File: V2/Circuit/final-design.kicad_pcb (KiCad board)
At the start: 2 copper layers, 62.8 x 62.2 mm, 27 parts, among them J1 Conn_02x05_Odd_Even, U1 LM338T, U2 TMC2209_SILENTSTEPSTICK

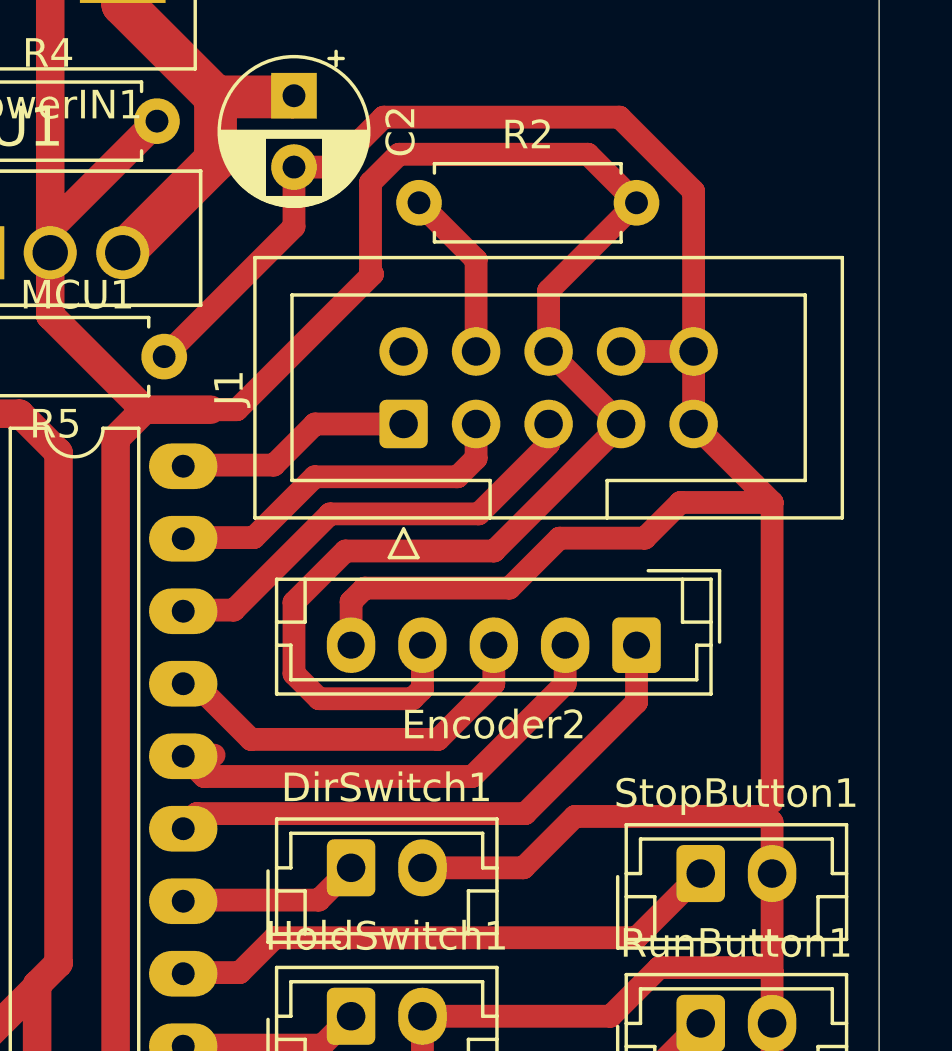
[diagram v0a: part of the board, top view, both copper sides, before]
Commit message: minor circuit changes
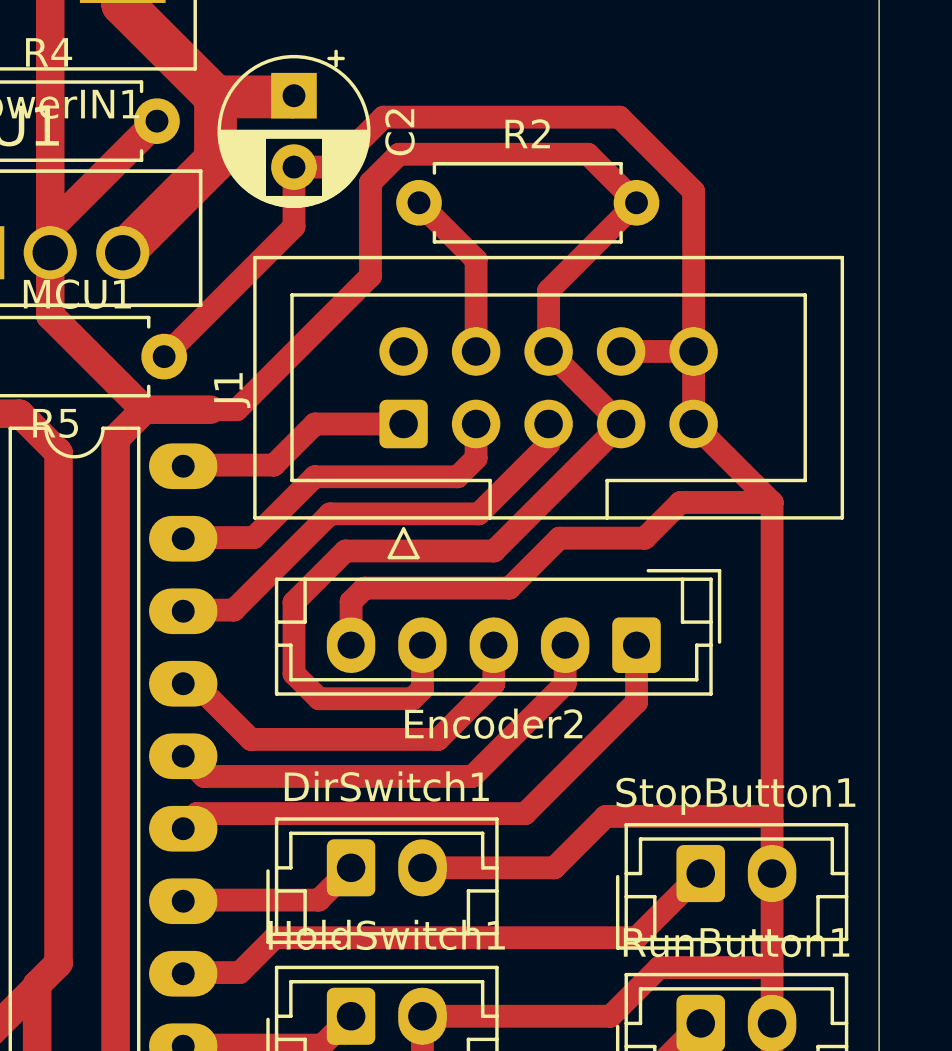
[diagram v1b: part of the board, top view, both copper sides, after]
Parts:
- R4: value 200 -> 150
- R5: value 330 -> 470
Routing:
- net Encoder_DT2: track 17.3 -> 16.2 mm
- net GND: track 356.7 -> 357.4 mm
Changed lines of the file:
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@@
 			)
 		)
-		(property "Value" "200"
+		(property "Value" "150"
 			(at 5.31 0 0)
 			(layer "F.Fab")
@@
 		)
 		(property "Value" "STC8H8K64U_SKDIP28"
-			(at 0.1 -21 0)
+			(at 0 0 90)
 			(unlocked yes)
 			(layer "F.Fab")
@@
 		)
 		(fp_text user "${REFERENCE}"
-			(at -0.2 -19.5 0)
+			(at 0.19 -15.99 0)
 			(unlocked yes)
 			(layer "F.Fab")
@@
 		)
 		(property "Value" "TMC2209_SILENTSTEPSTICK"
-			(at 11.05 11.115 0)
+			(at -1.15 -0.81 90)
 			(layer "F.Fab")
 			(effects
@@
 			)
 		)
-		(property "Value" "330"
+		(property "Value" "470"
 			(at 2.31 0 0)
 			(layer "F.Fab")
@@
 	)
 	(segment
-		(start 151.5 91.25)
-		(end 151.5 80.75)
-		(width 0.8)
-		(layer "F.Cu")
-		(net 1)
-	)
-	(segment
 		(start 121.529899 100.5)
 		(end 121.529899 100.499999)
@@
 	)
 	(segment
+		(start 151.3 91.75)
+		(end 145.669239 91.75)
+		(width 0.8)
+		(layer "F.Cu")
+		(net 1)
+	)
+	(segment
 		(start 146.75 114.25)
 		(end 146.25 114.75)
@@
 	)
 	(segment
-		(start 151.5 93.75)
-		(end 151.5 91.95)
+		(start 145.669239 91.75)
+		(end 143.869239 93.55)
 		(width 0.8)
 		(layer "F.Cu")
@@
 	)
 	(segment
-		(start 144.588478 91.75)
-		(end 142.788478 93.55)
-		(width 0.8)
-		(layer "F.Cu")
-		(net 1)
-	)
-	(segment
 		(start 105.916 95.166)
 		(end 104.95 94.2)
@@
 	)
 	(segment
+		(start 151.5 91.95)
+		(end 151.3 91.75)
+		(width 0.8)
+		(layer "F.Cu")
+		(net 1)
+	)
+	(segment
 		(start 119.75 113)
 		(end 122.69 113)
@@
 	)
 	(segment
+		(start 151.5 91.95)
+		(end 151.5 80.75)
+		(width 0.8)
+		(layer "F.Cu")
+		(net 1)
+	)
+	(segment
 		(start 104.05 76.34)
 		(end 105.65 74.74)
@@
 	)
 	(segment
-		(start 151.3 91.75)
-		(end 144.588478 91.75)
+		(start 134.75 69)
+		(end 136.137358 69)
 		(width 0.8)
 		(layer "F.Cu")
@@
 	)
 	(segment
-		(start 151.5 91.95)
-		(end 151.3 91.75)
+		(start 136.75 84.225)
+		(end 137.225 83.75)
 		(width 0.8)
 		(layer "F.Cu")
@@
 	)
 	(segment
-		(start 142.788478 93.55)
+		(start 143.869239 93.55)
 		(end 139.25 93.55)
 		(width 0.8)
@@
 	)
 	(segment
-		(start 134.75 69)
-		(end 136.137358 69)
-		(width 0.8)
-		(layer "F.Cu")
-		(net 1)
-	)
-	(segment
-		(start 136.75 84.225)
-		(end 137.225 83.75)
-		(width 0.8)
-		(layer "F.Cu")
-		(net 1)
-	)
-	(segment
 		(start 148.75 75.46)
 		(end 146.21 75.46)
@@
 	)
 	(segment
+		(start 151.5 93.75)
+		(end 151.5 91.95)
+		(width 0.8)
+		(layer "F.Cu")
+		(net 1)
+	)
+	(segment
 		(start 105.916 99.342956)
 		(end 105.916 95.166)
@@
 	)
 	(segment
+		(start 146.75 70.25)
+		(end 145.05 68.55)
+		(width 0.8)
+		(layer "F.Cu")
+		(net 14)
+	)
+	(segment
 		(start 104.065 70.35)
 		(end 104.065 69.159874)
@@
 	)
 	(segment
+		(start 145.05 68.55)
+		(end 138.425836 68.55)
+		(width 0.8)
+		(layer "F.Cu")
+		(net 14)
+	)
+	(segment
 		(start 141.76 82.45)
 		(end 136.55 82.45)
@@
 	)
 	(segment
-		(start 137.5 72.75)
-		(end 132.75 77.5)
-		(width 0.8)
-		(layer "F.Cu")
-		(net 14)
-	)
-	(segment
 		(start 121.17 62.70868)
 		(end 121.17 60.714466)
@@
 	)
 	(segment
-		(start 146.75 70.25)
-		(end 145.05 68.55)
-		(width 0.8)
-		(layer "F.Cu")
-		(net 14)
-	)
-	(segment
 		(start 122.62 107.38)
 		(end 123.23 107.38)
@@
 	)
 	(segment
-		(start 132.75 77.5)
-		(end 131.834415 77.5)
-		(width 0.8)
+		(start 117.87868 66)
+		(end 121.17 62.70868)
+		(width 1)
 		(layer "F.Cu")
 		(net 14)
 	)
 	(segment
-		(start 145.05 68.55)
-		(end 138.425836 68.55)
+		(start 138.425836 68.55)
+		(end 137.43 69.545836)
 		(width 0.8)
 		(layer "F.Cu")
@@
 	)
 	(segment
-		(start 117.87868 66)
-		(end 121.17 62.70868)
-		(width 1)
-		(layer "F.Cu")
-		(net 14)
-	)
-	(segment
 		(start 122.634466 59.25)
 		(end 124.705534 59.25)
@@
 	)
 	(segment
-		(start 104.065 69.159874)
-		(end 107.224874 66)
-		(width 1)
+		(start 137.43 72.82)
+		(end 132.75 77.5)
+		(width 0.8)
 		(layer "F.Cu")
 		(net 14)
 	)
 	(segment
-		(start 138.425836 68.55)
-		(end 137.43 69.545836)
-		(width 0.8)
+		(start 104.065 69.159874)
+		(end 107.224874 66)
+		(width 1)
 		(layer "F.Cu")
 		(net 14)
@@
 	)
 	(segment
-		(start 137.43 72.68)
-		(end 137.5 72.75)
-		(width 0.8)
-		(layer "F.Cu")
-		(net 14)
-	)
-	(segment
 		(start 124.705534 59.25)
 		(end 126.21 60.754466)
@@
 	)
 	(segment
+		(start 137.43 69.545836)
+		(end 137.43 72.82)
+		(width 0.8)
+		(layer "F.Cu")
+		(net 14)
+	)
+	(segment
 		(start 126.21 71.13)
 		(end 129.95 67.39)
@@
 	)
 	(segment
-		(start 137.43 69.545836)
-		(end 137.43 72.68)
+		(start 132.75 77.5)
+		(end 131.834415 77.5)
 		(width 0.8)
 		(layer "F.Cu")
@@
 	)
 	(segment
-		(start 130.85 89.6)
-		(end 131.951522 89.6)
-		(width 0.8)
-		(layer "F.Cu")
-		(net 15)
-	)
-	(segment
